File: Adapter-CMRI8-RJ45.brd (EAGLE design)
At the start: 30.9 x 39.5 mm, 5 parts, among them J1 RJ45

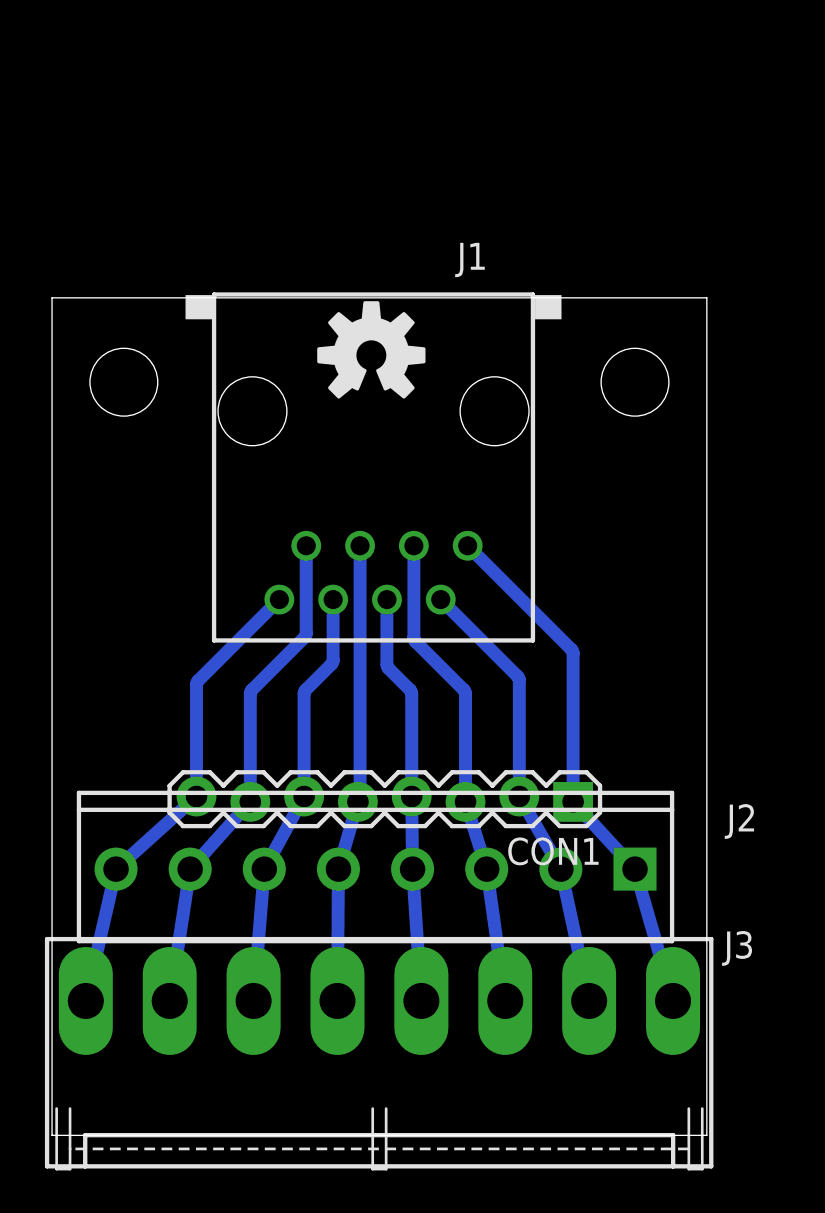
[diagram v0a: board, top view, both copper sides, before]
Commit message: 4.0
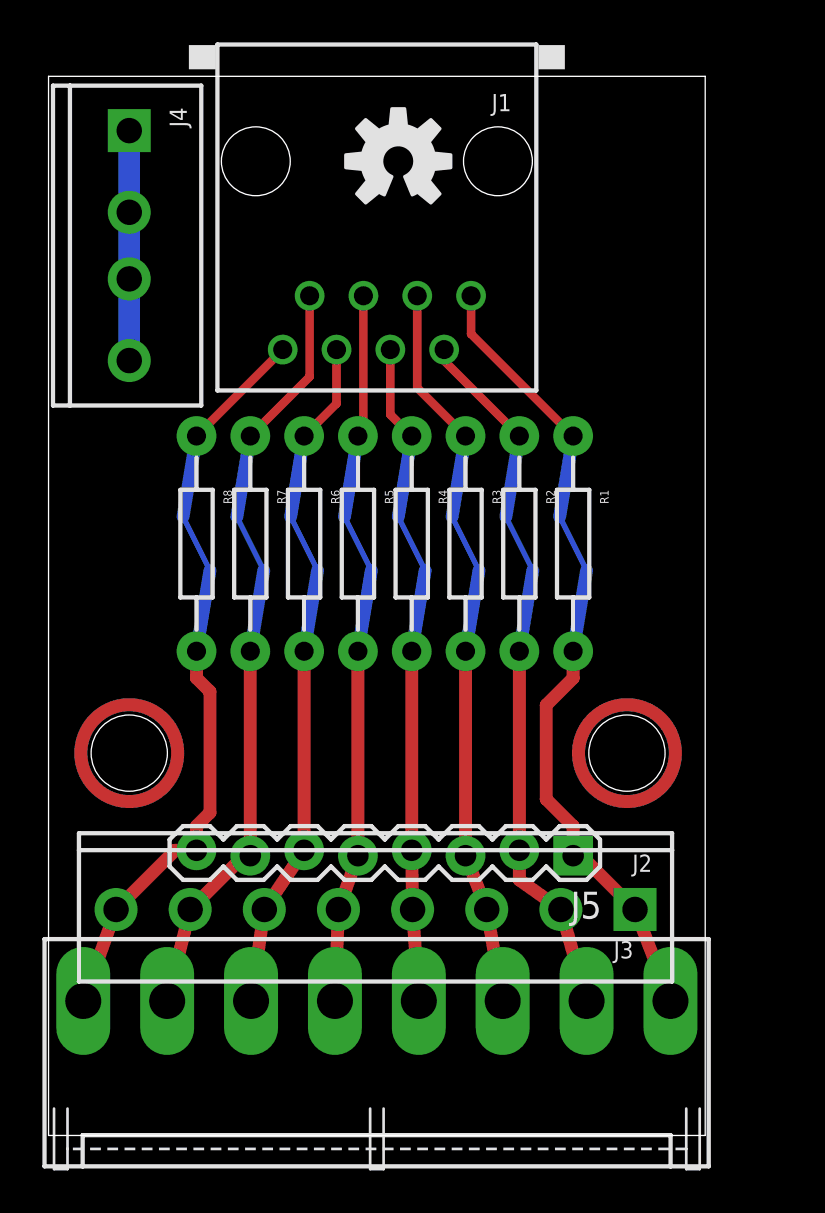
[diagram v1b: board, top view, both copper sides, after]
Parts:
- removed CON1: (no value), SPCoast:1X08_LOCK
- added J4: (no value), SPCoast:SCREWTERMINAL-3.5MM-4_LOCK
- added J5: (no value), SPCoast:1X08_LOCK
- added M1, M2: MOUNTINGHOLE, SPCoast:MOUNTINGHOLE
- added R1, R2, R3, R4, R5, R6, R7, R8: (no value), SPCoast:AXIAL-0.4-RES
- U$1: value OSHW-LOGOM -> DOC-OSHW-LOGO-M; device SparkFun:OSHW-LOGO-M -> SPCoast:OSHW-LOGO-M
- moved J1 11.8 mm to (15.5, 46.0)
- moved U$1 9.25 mm to (16.5, 46.0)
- moved J2 1.91 mm to (27.7, 10.7)
- moved J3 0.12 mm to (15.5, 6.35)
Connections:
- new net GND: J4.1, J4.2, J4.3, J4.4
- net L1: now also J5.1, R1.P$1, R1.P$2; no longer CON1.1
- net L2: now also J5.2, R2.P$1, R2.P$2; no longer CON1.2
- net L3: now also J5.3, R3.P$1, R3.P$2; no longer CON1.3
- net L4: now also J5.4, R4.P$1, R4.P$2; no longer CON1.4
- net L5: now also J5.5, R5.P$1, R5.P$2; no longer CON1.5
- net L6: now also J5.6, R6.P$1, R6.P$2; no longer CON1.6
- net L7: now also J5.7, R7.P$1, R7.P$2; no longer CON1.7
- net L8: now also J5.8, R8.P$1, R8.P$2; no longer CON1.8
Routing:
- net L1: track 24.9 -> 38.5 mm
- net L8: track 22.4 -> 35.8 mm
- net L3: track 22.7 -> 35.7 mm
- net L2: track 21.1 -> 33.8 mm
- net L7: track 23.7 -> 36.3 mm
- net L6: track 20.0 -> 32.4 mm
- net L5: track 21.7 -> 34.0 mm
- net L4: track 19.4 -> 31.6 mm
- net GND: track 0.00 -> 10.9 mm
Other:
- board size 30.9 x 39.5 mm -> 31 x 50 mm
- board text added: "0.156""
- board text added: "2018.12"
- board text added: "COMMON"
- board text added: "Cut on reverse for Resistors"
- board text added: "J1"
- board text added: "J2"
- board text added: "J3"
- board text added: "J4"
- board text added: "J5"
- board text added: "MRCS"
- board text added: "R1"
- board text added: "R2"
- board text added: "R3"
- board text added: "R4"
- board text added: "R5"
- board text added: "R6"
- board text added: "R7"
- board text added: "R8"
- board text added: "Resistor"
- board text added: "Tie points"
- board text added: "v4.0"
- board text added: "www . SPCoast . com"
- board text removed: ".com"
- board text removed: "2017.11"
- board text removed: "Lines"
- board text removed: "SP Coast"
- board text removed: "Shore"
- board text removed: "South"
- board text removed: "v3.0"
- board text removed: "www."
